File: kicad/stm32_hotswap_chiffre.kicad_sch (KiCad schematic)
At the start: 24 parts, among them J1 USB_C_Receptacle_USB2.0, J2 OLED I2C, J3 SW_DEBUG, U2 STM32F072CBT6, U3 USBLC6-2SC6

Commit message: more bom work
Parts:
- C? (x5), R? (x2): JlcRotOffset (none) -> 90
- D100: JlcRotOffset (none) -> 0
- J1: JlcPosOffset (none) -> 0,1.5; JlcRotOffset (none) -> 180
- U2, U?: JlcRotOffset (none) -> 180
- U3: JlcRotOffset (none) -> -90; LCSC (none) -> C2827654
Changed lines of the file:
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@@
+      (effects (font (size 1.27 1.27)) hide)
+    )
+    (property "JlcRotOffset" "180" (at 154.94 48.26 0)
+      (effects (font (size 1.27 1.27)) hide)
+    )
+    (property "JlcPosOffset" "0,1.5" (at 154.94 48.26 0)
       (effects (font (size 1.27 1.27)) hide)
     )
@@
       (effects (font (size 1.27 1.27)) hide)
     )
+    (property "JlcRotOffset" "0" (at 212.725 107.95 0)
+      (effects (font (size 1.27 1.27)) hide)
+    )
     (pin "1")
     (pin "2")
@@
     )
     (property "Datasheet" "https://www.st.com/resource/en/datasheet/usblc6-2.pdf" (at 171.45 96.52 0)
+      (effects (font (size 1.27 1.27)) hide)
+    )
+    (property "LCSC" "C2827654" (at 166.37 105.41 0)
+      (effects (font (size 1.27 1.27)) hide)
+    )
+    (property "JlcRotOffset" "-90" (at 166.37 105.41 0)
       (effects (font (size 1.27 1.27)) hide)
     )
@@
       (effects (font (size 1.27 1.27)) hide)
     )
+    (property "JlcRotOffset" "90" (at 90.17 108.585 0)
+      (effects (font (size 1.27 1.27)) hide)
+    )
     (pin "1")
     (pin "2")
@@
     )
     (property "Datasheet" "https://www.st.com/resource/en/datasheet/stm32f072cb.pdf" (at 41.275 72.39 0)
+      (effects (font (size 1.27 1.27)) hide)
+    )
+    (property "JlcRotOffset" "180" (at 41.275 72.39 0)
       (effects (font (size 1.27 1.27)) hide)
     )
@@
       (effects (font (size 1.27 1.27)) hide)
     )
+    (property "JlcRotOffset" "90" (at 116.84 69.85 0)
+      (effects (font (size 1.27 1.27)) hide)
+    )
     (pin "1")
     (pin "2")
@@
       (effects (font (size 1.27 1.27)) hide)
     )
+    (property "JlcRotOffset" "180" (at 106.68 36.83 0)
+      (effects (font (size 1.27 1.27)) hide)
+    )
     (pin "1")
     (pin "2")
@@
       (effects (font (size 1.27 1.27)) hide)
     )
+    (property "JlcRotOffset" "90" (at 105.41 69.85 0)
+      (effects (font (size 1.27 1.27)) hide)
+    )
     (pin "1")
     (pin "2")
@@
       (effects (font (size 1.27 1.27)) hide)
     )
+    (property "JlcRotOffset" "90" (at 82.55 69.85 0)
+      (effects (font (size 1.27 1.27)) hide)
+    )
     (pin "1")
     (pin "2")
@@
       (effects (font (size 1.27 1.27)) hide)
     )
+    (property "JlcRotOffset" "90" (at 128.27 69.85 0)
+      (effects (font (size 1.27 1.27)) hide)
+    )
     (pin "1")
     (pin "2")
@@
       (effects (font (size 1.27 1.27)) hide)
     )
+    (property "JlcRotOffset" "90" (at 93.98 69.85 0)
+      (effects (font (size 1.27 1.27)) hide)
+    )
     (pin "1")
     (pin "2")
@@
       (effects (font (size 1.27 1.27)) hide)
     )
+    (property "JlcRotOffset" "90" (at 90.17 118.745 0)
+      (effects (font (size 1.27 1.27)) hide)
+    )

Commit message: update 3d models
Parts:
- SW? (x2): footprint Button_Switch_SMD:SW_SPST_SKQG_WithoutStem -> modified_footrprints:SW_SPST_SKQG_WithoutStem
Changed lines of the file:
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@@
       (effects (font (size 1.27 1.27)))
     )
-    (property "Footprint" "Button_Switch_SMD:SW_SPST_SKQG_WithoutStem" (at 121.92 97.155 0)
+    (property "Footprint" "modified_footrprints:SW_SPST_SKQG_WithoutStem" (at 121.92 97.155 0)
       (effects (font (size 1.27 1.27)) hide)
     )
@@
       (effects (font (size 1.27 1.27)))
     )
-    (property "Footprint" "Button_Switch_SMD:SW_SPST_SKQG_WithoutStem" (at 96.52 99.695 0)
-      (effects (font (size 1.27 1.27)) hide)
-    )
+    (property "Footprint" "modified_footrprints:SW_SPST_SKQG_WithoutStem" (at 96.52 99.695 0)
+      (effects (font (size 1.27 1.27)) hide)
+    )

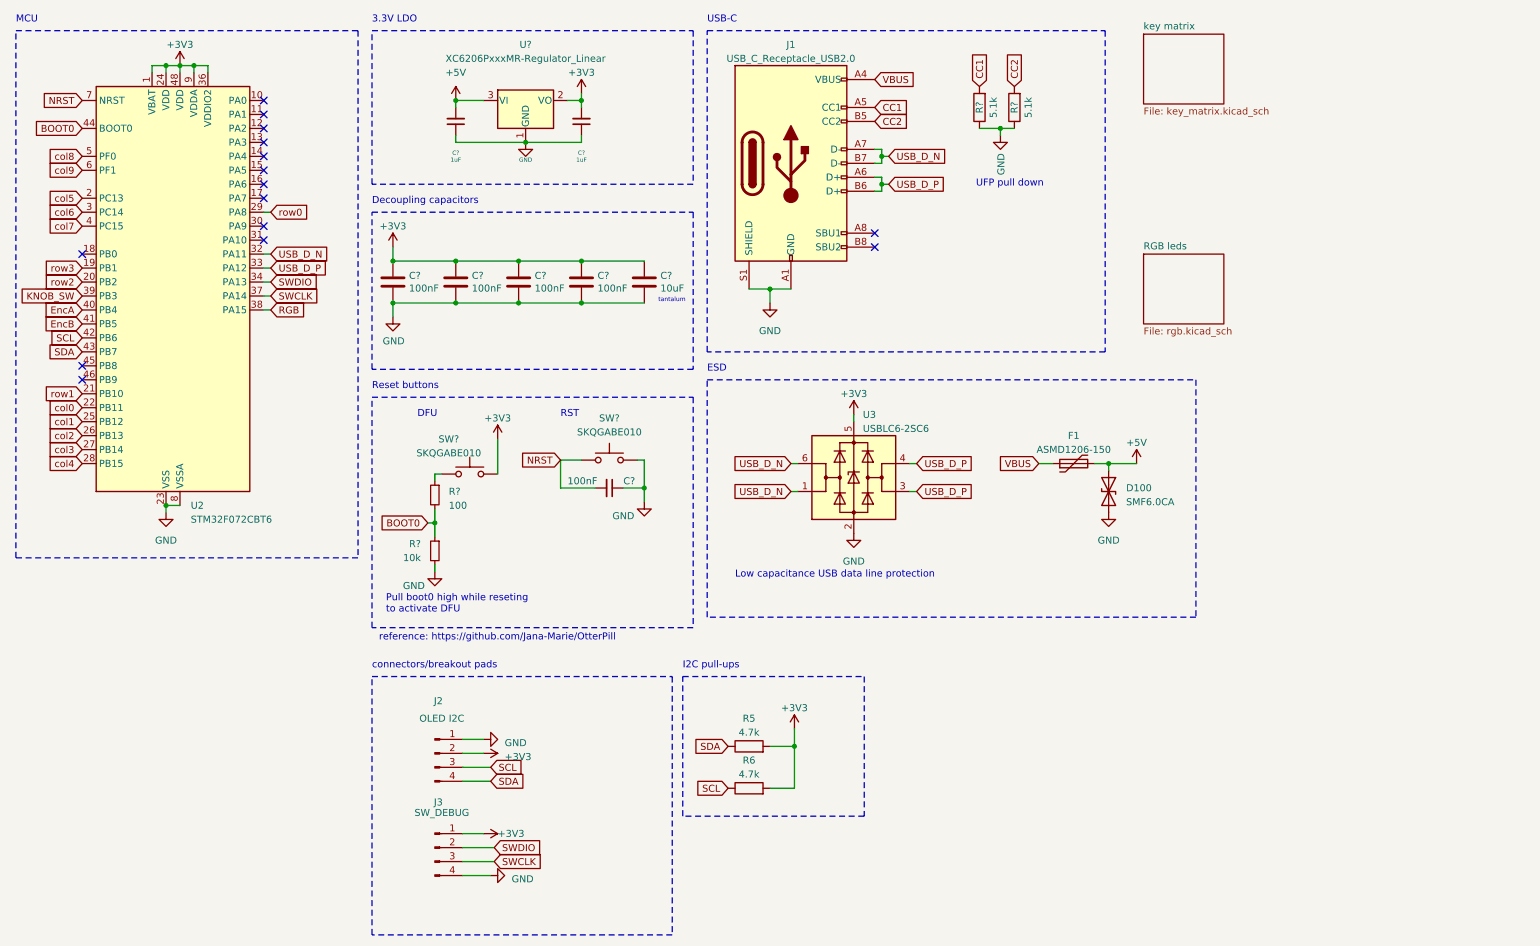
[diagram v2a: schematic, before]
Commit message: esd and usb update/
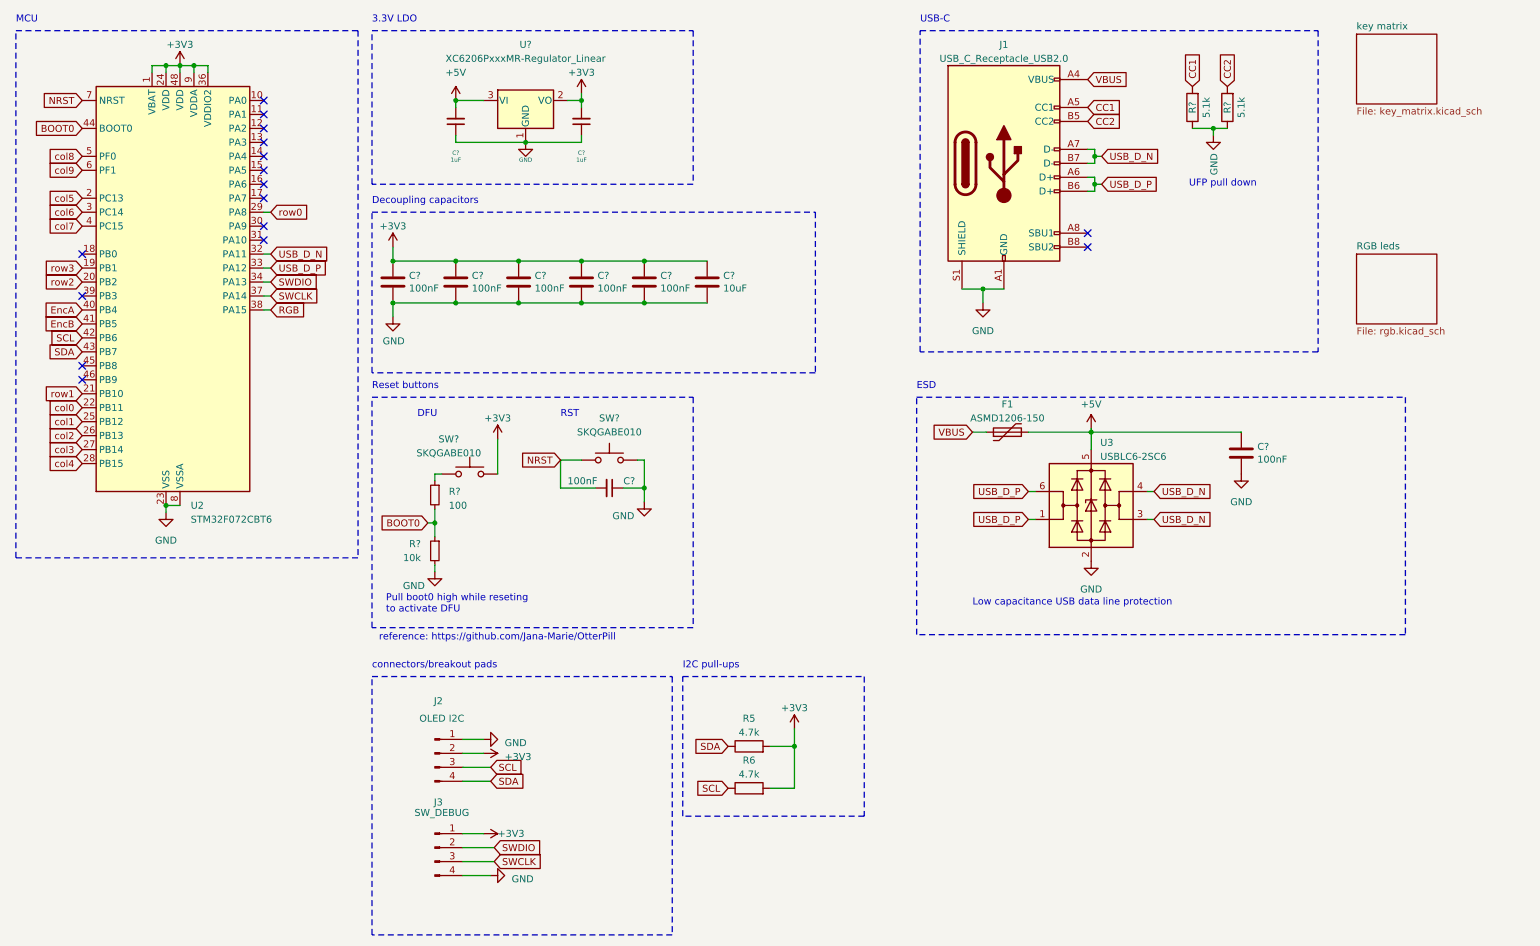
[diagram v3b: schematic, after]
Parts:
- removed D100: SMF6.0CA, Diode_SMD:D_SOD-123F, symbol Device:D_TVS
- added C? (x2): 100nF, Capacitor_SMD:C_0402_1005Metric, symbol Device:C
- C?: footprint Capacitor_Tantalum_SMD:CP_EIA-3216-18_Kemet-A -> Capacitor_SMD:C_0603_1608Metric; LCSC C7171 -> (none)
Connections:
- net +3V3: now also C?.1; no longer U3.5 (VBUS)
- net +5V: now also U3.5 (VBUS), C?.1
- net GND: now also C?.2, C?.2
- net USB_D_N: now also U3.3 (I/O2), U3.4 (I/O2); no longer U3.1 (I/O1), U3.6 (I/O1)
- net USB_D_P: now also U3.1 (I/O1), U3.6 (I/O1); no longer U3.3 (I/O2), U3.4 (I/O2)
- net KNOB_SW: no longer names the net of U2.39 (PB3)
- no-connect marks 15 -> 16
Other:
- note removed: "tantalum"
- moved on the sheet: C?, F1, J1, R?, U3

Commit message: cleaning up pcb
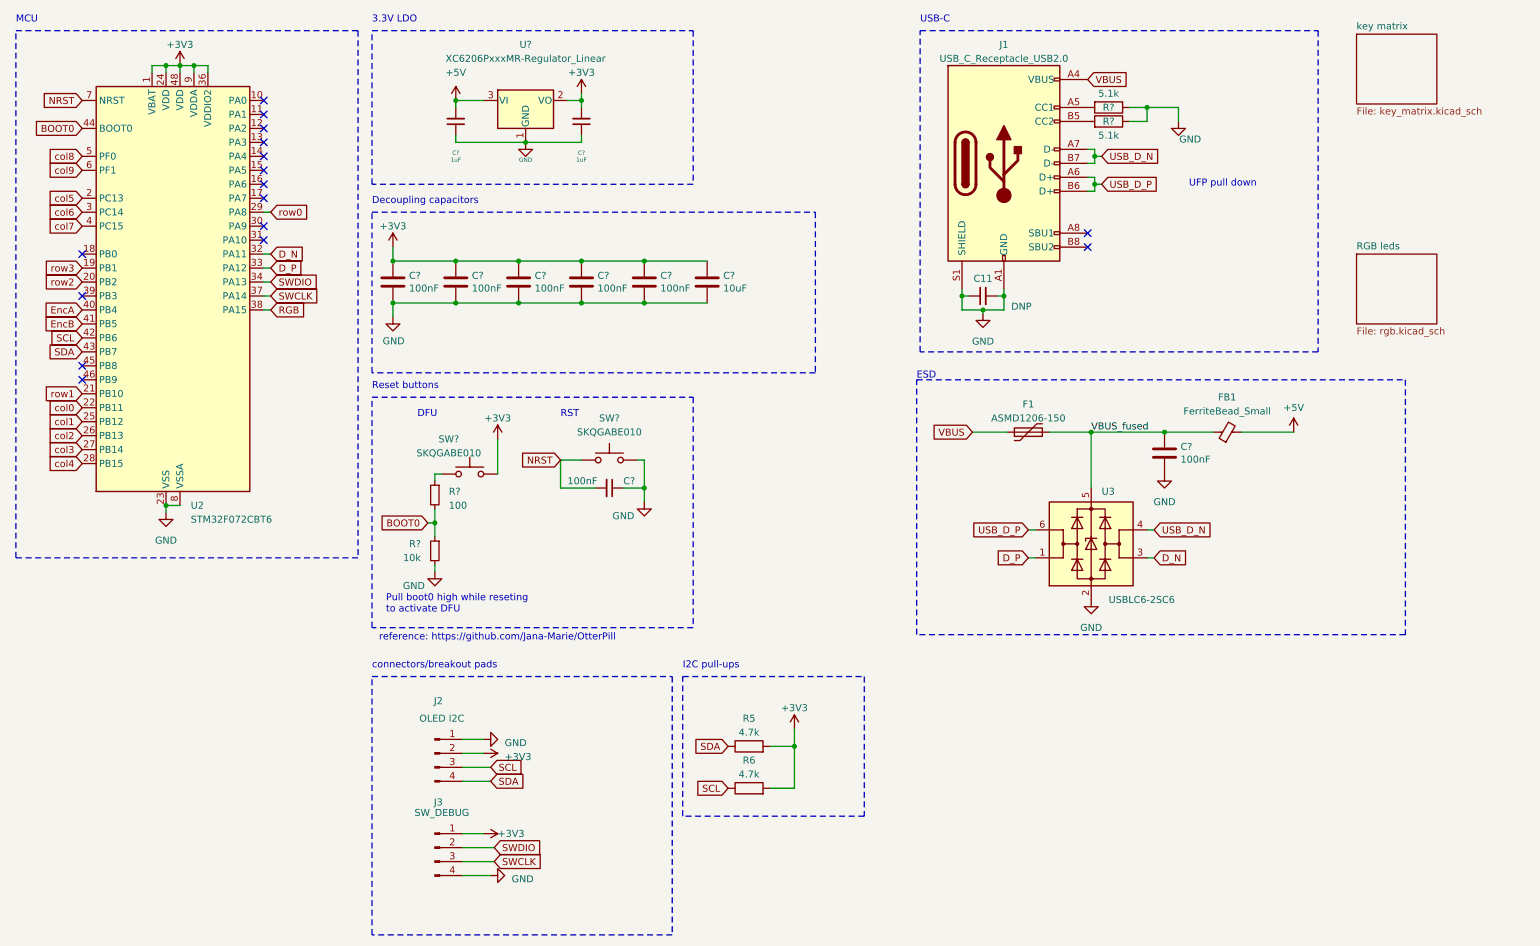
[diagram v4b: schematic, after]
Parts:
- added C11: DNP, Capacitor_SMD:C_0402_1005Metric, symbol Device:C_Small
- added FB1: FerriteBead_Small, Inductor_SMD:L_0805_2012Metric, symbol Device:FerriteBead_Small
- C?: now left out of the parts list
- R5, R6, R? (x4): footprint Resistor_SMD:R_0603_1608Metric -> Resistor_SMD:R_0402_1005Metric
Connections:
- net +5V: now also FB1.2; no longer C?.1, F1.2, U3.5 (VBUS)
- net GND: now also C11.1, C11.2
- net USB_D_N: no longer U2.32 (PA11), U3.3 (I/O2)
- net USB_D_P: no longer U2.33 (PA12), U3.1 (I/O1)
- net CC1: no longer names the net of J1.A5 (CC1)
- net CC1: now also R?.2; no longer R?.2
- net CC2: no longer names the net of J1.B5 (CC2)
- net CC2: now also R?.2; no longer R?.2
- new net D_N: U2.32 (PA11), U3.3 (I/O2)
- new net D_P: U2.33 (PA12), U3.1 (I/O1)
- new net VBUS_fused: C?.1, F1.2, FB1.1, U3.5 (VBUS)
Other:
- note removed: "Low capacitance USB data line protection"
- moved on the sheet: C?, F1, R?, U3

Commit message: v0.2
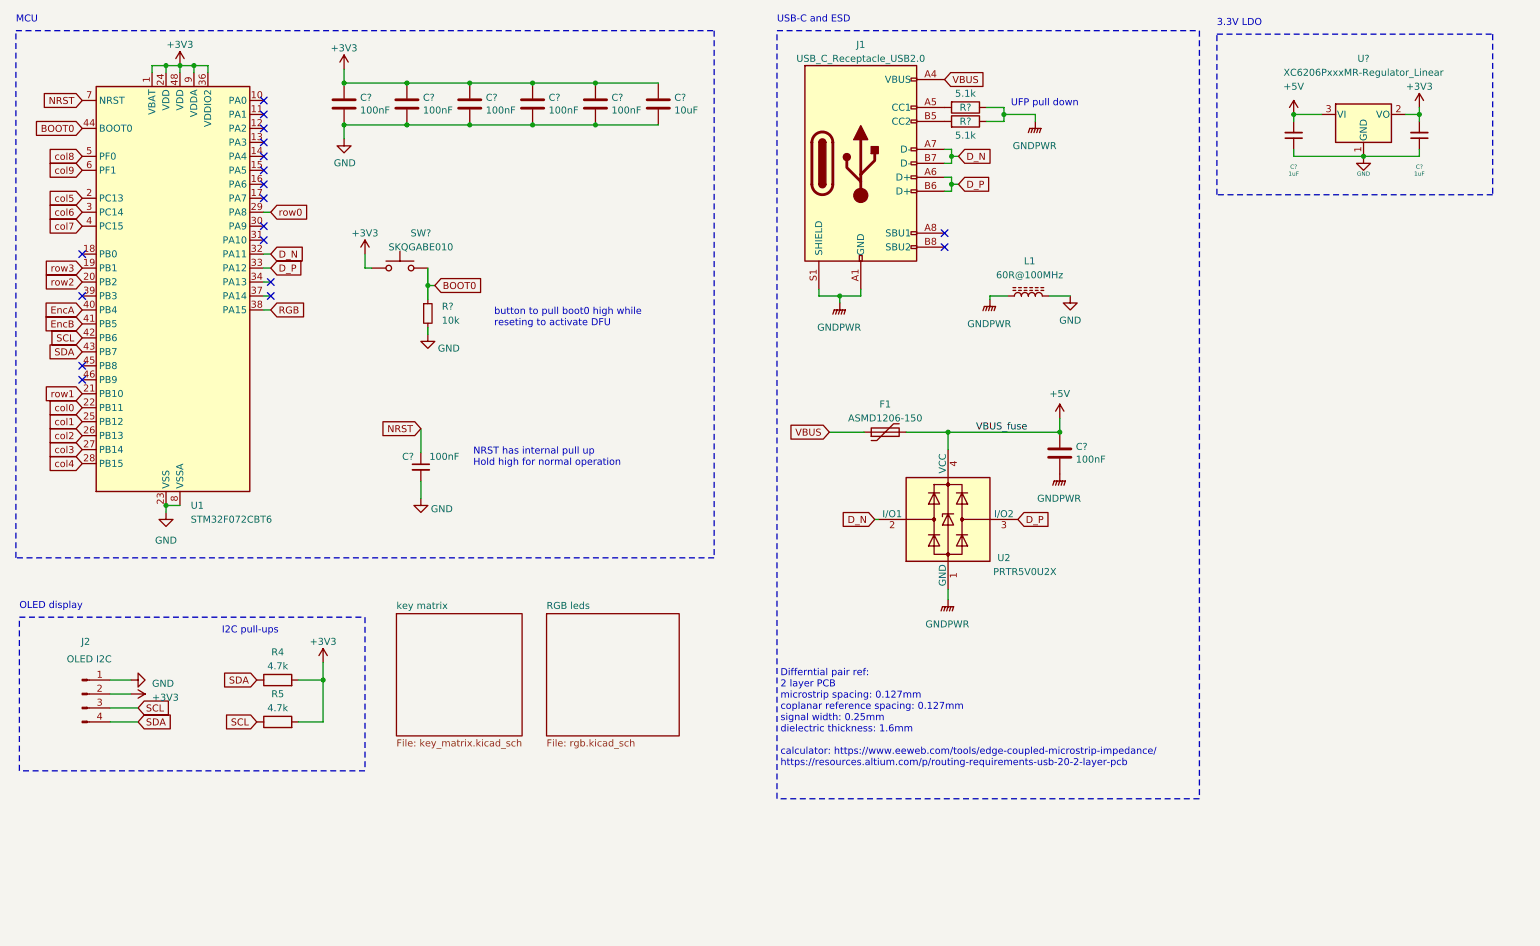
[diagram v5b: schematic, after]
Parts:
- removed C11: DNP, Capacitor_SMD:C_0402_1005Metric, symbol Device:C_Small
- removed FB1: FerriteBead_Small, Inductor_SMD:L_0805_2012Metric, symbol Device:FerriteBead_Small
- removed J3: SW_DEBUG, Connector_PinHeader_2.54mm:PinHeader_1x04_P2.54mm_Vertical, symbol Connector:Conn_01x04_Pin
- removed R?: 100, Resistor_SMD:R_0402_1005Metric, symbol Device:R_Small
- removed SW?: SKQGABE010, modified_footrprints:SW_SPST_SKQG_WithoutStem, symbol Switch:SW_Push
- removed U3: USBLC6-2SC6, Package_TO_SOT_SMD:SOT-23-6, symbol Power_Protection:USBLC6-2SC6
- added L1: 60R@100MHz, Inductor_SMD:L_1206_3216Metric, symbol Unified-Daughterboard-rescue:L_Core_Ferrite-Device
- added U2: PRTR5V0U2X, Package_TO_SOT_SMD:SOT-143, symbol Power_Protection:PRTR5V0U2X
- C?: now in the parts list
- C? (x7), R?: JlcRotOffset 90 -> (none)
- F1: LCSC (none) -> C135341
- U1: renamed from U2; JlcRotOffset 180 -> 90
- U?: JlcRotOffset 180 -> (none)
- renumbered R5 to R4, R6 to R5
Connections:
- net USB_D_N is gone; now on net D_N: J1.A7 (D-), J1.B7 (D-)
- net USB_D_P is gone; now on net D_P: J1.A6 (D+), J1.B6 (D+)
- net VBUS_fused is gone; now on net +5V: C?.1, F1.2
- net +5V: now also U2.4 (VCC)
- net BOOT0: now also SW?.2
- net D_N: now also U2.2 (I/O1)
- net D_P: now also U2.3 (I/O2)
- net GND: now also C?.2, L1.2; no longer C?.1, C?.2, J1.A1 (GND), J1.A12 (GND), J1.B1 (GND), J1.B12 (GND), J1.S1 (SHIELD), R?.1, R?.1
- net NRST: now also C?.1; no longer C?.2
- net SWCLK: no longer names the net of U1.37 (PA14)
- net SWDIO: no longer names the net of U1.34 (PA13)
- new net GNDPWR: C?.2, J1.A1 (GND), J1.A12 (GND), J1.B1 (GND), J1.B12 (GND), J1.S1 (SHIELD), L1.1, R?.1, R?.1, U2.1 (GND)
- no-connect marks 16 -> 18
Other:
- note added: "Differntial pair ref: 2 layer PCB microstrip spacing: 0.127mm coplanar reference spacing: 0.127mm signal width: 0.25mm dielectric thickness: 1.6mm calculator: https://www.eeweb.com/tools/edge-coupled-microstrip-impedance/ https://resources.altium.com/p/routing-requirements-usb-20-2-layer-pcb"
- note added: "NRST has internal pull up Hold high for normal operation"
- note added: "OLED display"
- note added: "USB-C and ESD"
- note added: "button to pull boot0 high while reseting to activate DFU"
- note removed: "DFU"
- note removed: "Decoupling capacitors"
- note removed: "ESD"
- note removed: "Pull boot0 high while reseting to activate DFU"
- note removed: "RST"
- note removed: "Reset buttons"
- note removed: "USB-C"
- note removed: "connectors/breakout pads"
- note removed: "reference: https://github.com/Jana-Marie/OtterPill"
- moved on the sheet: C?, F1, J1, J2, R4, R5, R?, SW?, U?
